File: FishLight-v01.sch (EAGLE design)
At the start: 213 parts, among them Q1 RK7002BSOT23-3, Q10 RK7002BSOT23-3, Q11 RK7002BSOT23-3, Q12 RK7002BSOT23-3, Q13 RK7002BSOT23-3, Q14 RK7002BSOT23-3, Q15 RK7002BSOT23-3, Q2 RK7002BSOT23-3, Q3 RK7002BSOT23-3, Q4 RK7002BSOT23-3, Q5 RK7002BSOT23-3, Q6 RK7002BSOT23-3, Q7 RK7002BSOT23-3, Q8 RK7002BSOT23-3, Q9 RK7002BSOT23-3, U1 SPARK_CORECORE, U10 AD5248MSOP-10, U11 INA219SOT23-8, U12 INA219SOT23-8, U13 INA219SOT23-8, U14 INA219SOT23-8, U15 INA219SOT23-8, U16 MIC29300D2PAK-3, U17 L7805D2PAK-2, U22 AD5248MSOP-10, U23 CAT4101TO-263, U24 CAT4101TO-263, U25 CAT4101TO-263, U26 INA219SOT23-8, U27 INA219SOT23-8, U28 INA219SOT23-8, U29 CD74HC4067SSOP24, U3 CAT4101TO-263, U30 CD74HC4067SSOP24, U31 RELAY-SOLIDSTATEPTH, U32 RELAY-SOLIDSTATEPTH, U33 RELAY-SOLIDSTATEPTH, U34 NC7SZ373TSSOP-6, U35 NC7SZ373TSSOP-6, U36 NC7SZ373TSSOP-6, U37 NC7SZ373TSSOP-6, U38 NC7SZ373TSSOP-6, U39 NC7SZ373TSSOP-6, U4 CAT4101TO-263, U40 NC7SZ373TSSOP-6, U41 NC7SZ373TSSOP-6, U42 NC7SZ373TSSOP-6, U43 NC7SZ373TSSOP-6, U44 NC7SZ373TSSOP-6, U45 NC7SZ373TSSOP-6, U46 NC7SZ373TSSOP-6, U47 NC7SZ373TSSOP-6, U48 NC7SZ373TSSOP-6, U49 DS18B20USOP8, U5 CAT4101TO-263, U6 CAT4101TO-263, U7 CAT4101TO-263, U8 AD5248MSOP-10, U9 AD5248MSOP-10

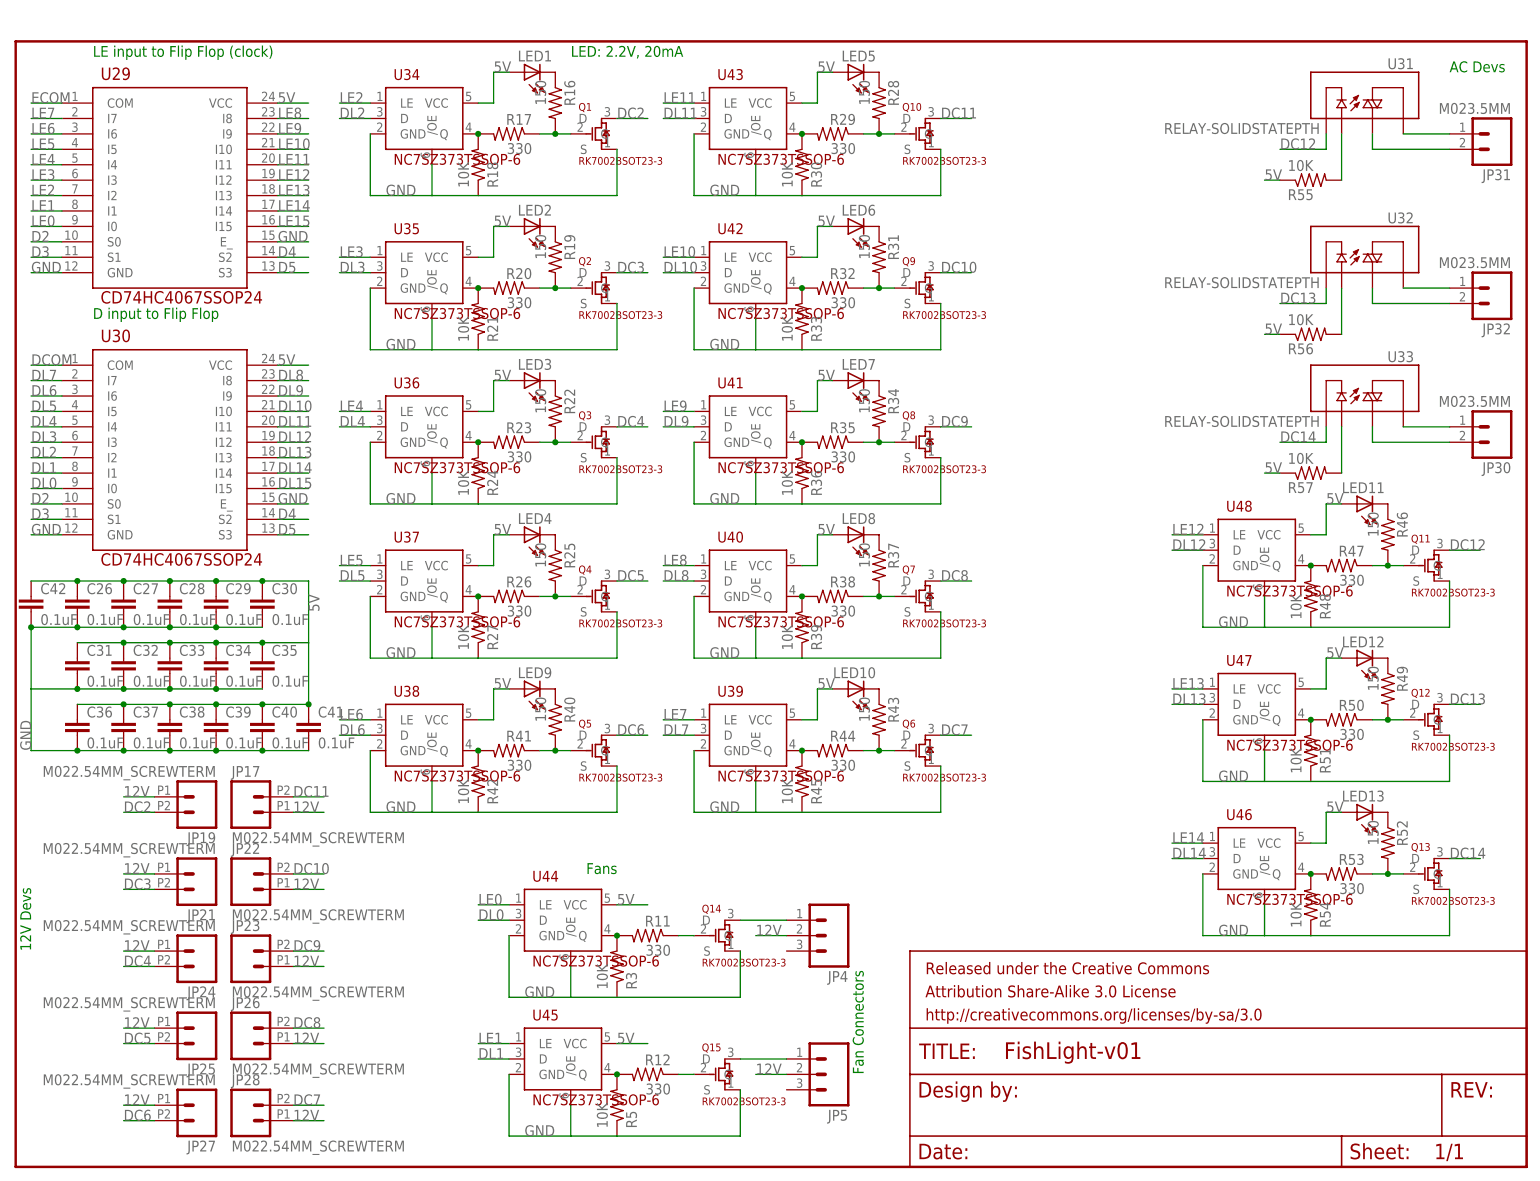
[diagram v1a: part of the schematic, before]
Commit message: FishLight_PCB: Changed 12V connectors
The old connectors were 2.54mm.  Changed to 3.5mm because they are
bigger, easier to use, and not as ugly either.  Also moved some
things around in order to get them to fit.
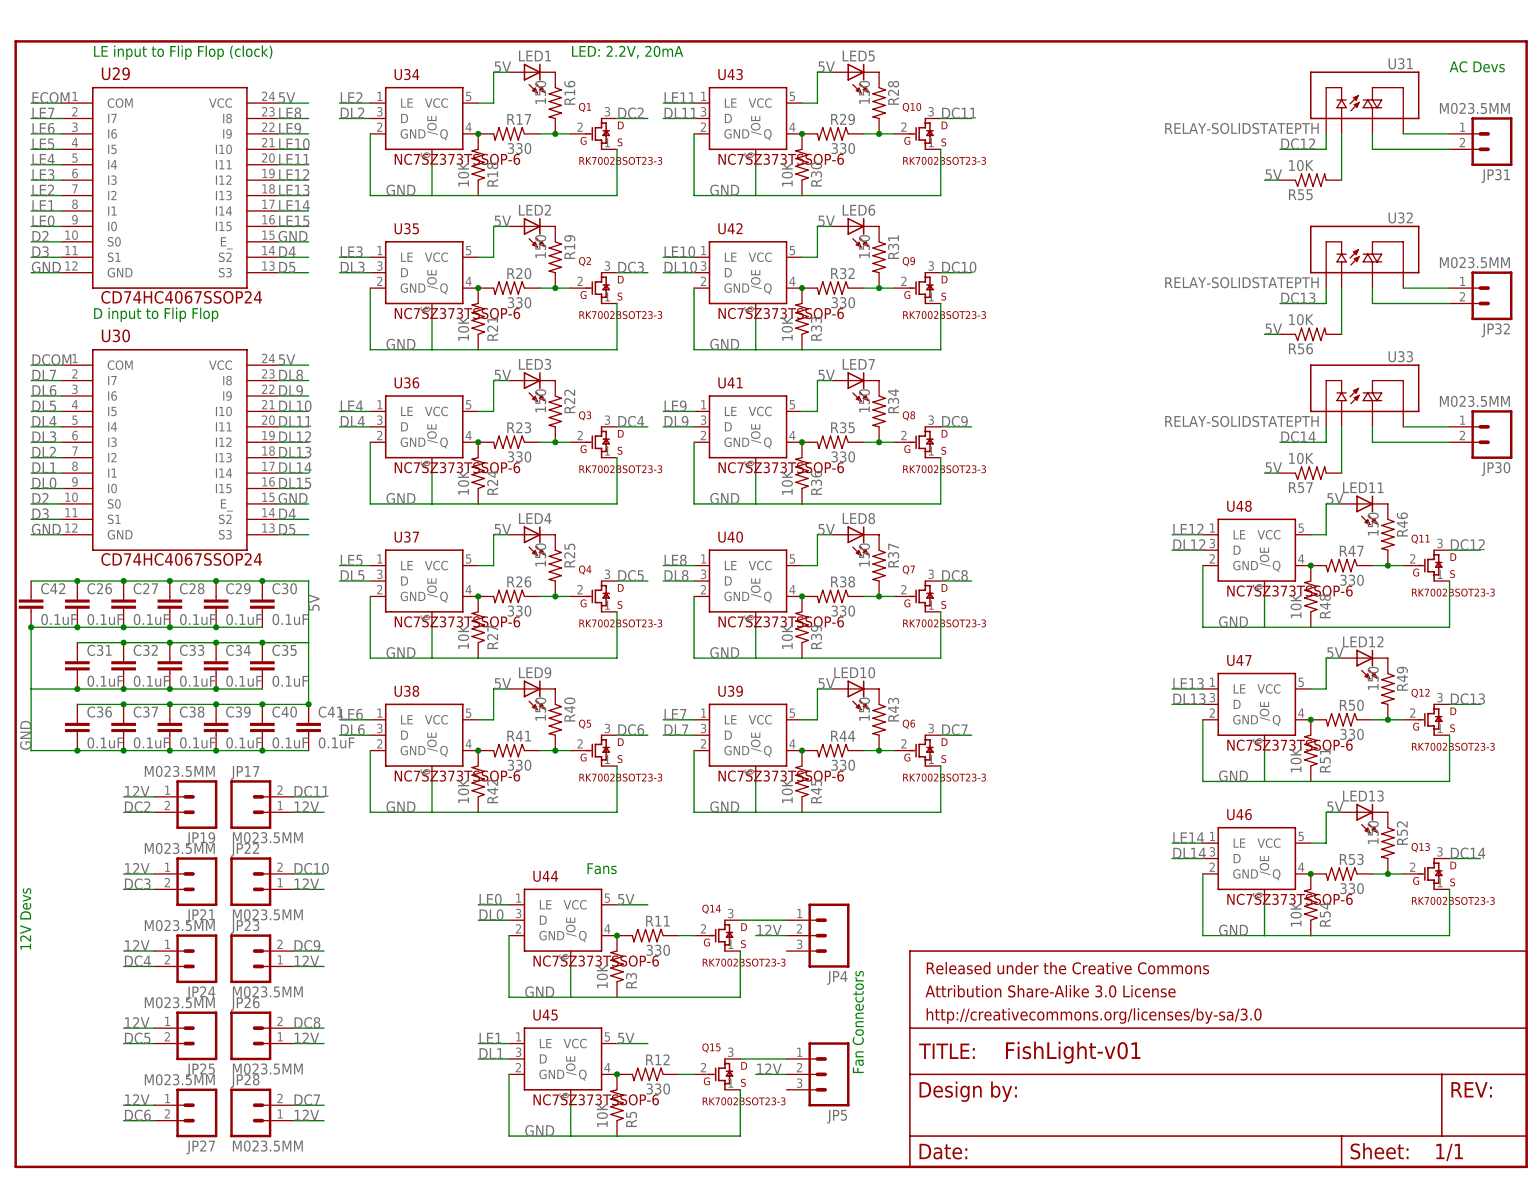
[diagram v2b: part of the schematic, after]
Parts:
- JP17, JP19, JP21, JP22, JP23, JP24, JP25, JP26, JP27, JP28: value M022.54MM_SCREWTERM -> M023.5MM; device Mikes-Stuff:M022.54MM_SCREWTERM -> Mikes-Stuff:M023.5MM
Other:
- moved on the sheet: Q1, Q10, Q11, Q12, Q13, Q14, Q15, Q2, Q3, Q4, Q5, Q6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
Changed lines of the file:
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@@
 <part name="C23" library="SparkFun-Capacitors" deviceset="0.1UF-25V(+80/-20%)(0603)" device="" value="0.1uF"/>
 <part name="C24" library="SparkFun-Capacitors" deviceset="0.1UF-25V(+80/-20%)(0603)" device="" value="0.1uF"/>
-<part name="JP17" library="Mikes-Stuff" deviceset="M02" device="2.54MM_SCREWTERM"/>
-<part name="JP19" library="Mikes-Stuff" deviceset="M02" device="2.54MM_SCREWTERM"/>
-<part name="JP21" library="Mikes-Stuff" deviceset="M02" device="2.54MM_SCREWTERM"/>
-<part name="JP22" library="Mikes-Stuff" deviceset="M02" device="2.54MM_SCREWTERM"/>
-<part name="JP23" library="Mikes-Stuff" deviceset="M02" device="2.54MM_SCREWTERM"/>
-<part name="JP24" library="Mikes-Stuff" deviceset="M02" device="2.54MM_SCREWTERM"/>
-<part name="JP25" library="Mikes-Stuff" deviceset="M02" device="2.54MM_SCREWTERM"/>
-<part name="JP26" library="Mikes-Stuff" deviceset="M02" device="2.54MM_SCREWTERM"/>
-<part name="JP27" library="Mikes-Stuff" deviceset="M02" device="2.54MM_SCREWTERM"/>
+<part name="JP17" library="Mikes-Stuff" deviceset="M02" device="3.5MM" value="M023.5MM"/>
+<part name="JP19" library="Mikes-Stuff" deviceset="M02" device="3.5MM" value="M023.5MM"/>
+<part name="JP21" library="Mikes-Stuff" deviceset="M02" device="3.5MM" value="M023.5MM"/>
+<part name="JP22" library="Mikes-Stuff" deviceset="M02" device="3.5MM" value="M023.5MM"/>
+<part name="JP23" library="Mikes-Stuff" deviceset="M02" device="3.5MM" value="M023.5MM"/>
+<part name="JP24" library="Mikes-Stuff" deviceset="M02" device="3.5MM" value="M023.5MM"/>
+<part name="JP25" library="Mikes-Stuff" deviceset="M02" device="3.5MM" value="M023.5MM"/>
+<part name="JP26" library="Mikes-Stuff" deviceset="M02" device="3.5MM" value="M023.5MM"/>
+<part name="JP27" library="Mikes-Stuff" deviceset="M02" device="3.5MM" value="M023.5MM"/>
 <part name="R11" library="SparkFun-Resistors" deviceset="RESISTOR" device="0603" value="330"/>
 <part name="FRAME2" library="SparkFun-Aesthetics" deviceset="FRAME-LETTER" device=""/>
@@
 <part name="R44" library="SparkFun-Resistors" deviceset="RESISTOR" device="0603" value="330"/>
 <part name="R45" library="SparkFun-Resistors" deviceset="RESISTOR" device="0603-RES" value="10K"/>
-<part name="JP28" library="Mikes-Stuff" deviceset="M02" device="2.54MM_SCREWTERM"/>
+<part name="JP28" library="Mikes-Stuff" deviceset="M02" device="3.5MM" value="M023.5MM"/>
 <part name="U48" library="Mikes-Stuff" deviceset="NC7SZ373" device="TSSOP-6"/>
 <part name="Q11" library="Mikes-Stuff" deviceset="RK7002B" device="SOT23-3"/>
